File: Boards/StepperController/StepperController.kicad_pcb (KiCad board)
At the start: 2 copper layers, 164 parts, among them IC1 ATMEGA645A-A, J1 I2C, J2 SPI_Extern, J3 ISP, J4 Reference, J5 Display, J7 Spindle, P1 Power, P10 CONN_Z, P2 Cover, P3 USB_B, P4 Relay2, P5 Relay1, P6 Emer_Off, P8 CONN_X, P9 CONN_Y, Q1 BC817-40, Q2 BC817-40, Q3 BC817-40, Q4 BC817-40, Q5 BC817-40, SW2 SW_1, SW3 SW_2, U1 LM2595S-5, U2 74LS11, U3 FT232RL, U5 TMC2660, U6 TMC2660, U7 TMC2660, U8 74HC00, X1 16MHz, Y1 20MHz

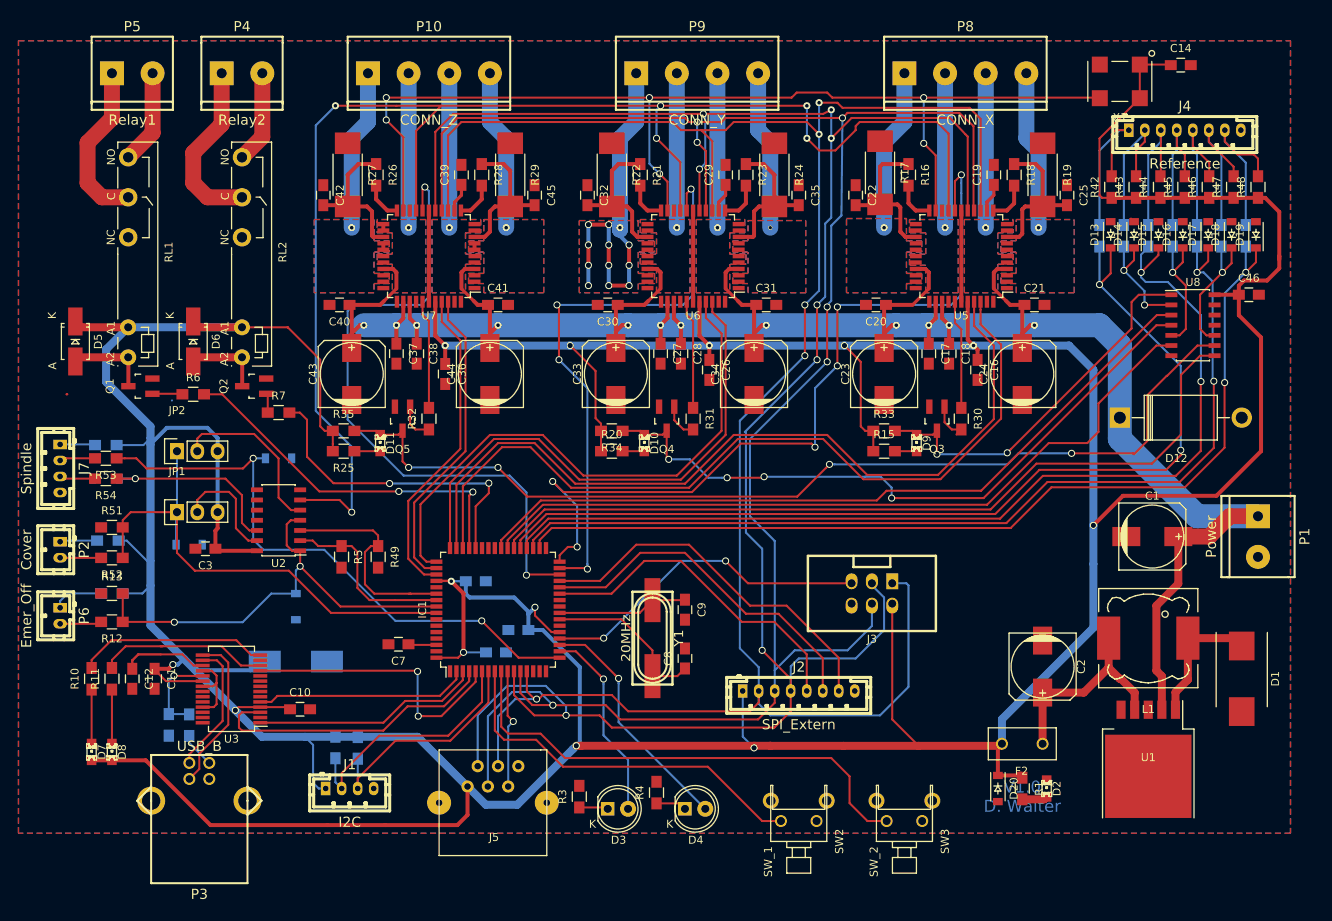
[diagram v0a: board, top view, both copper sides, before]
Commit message: Layouting...
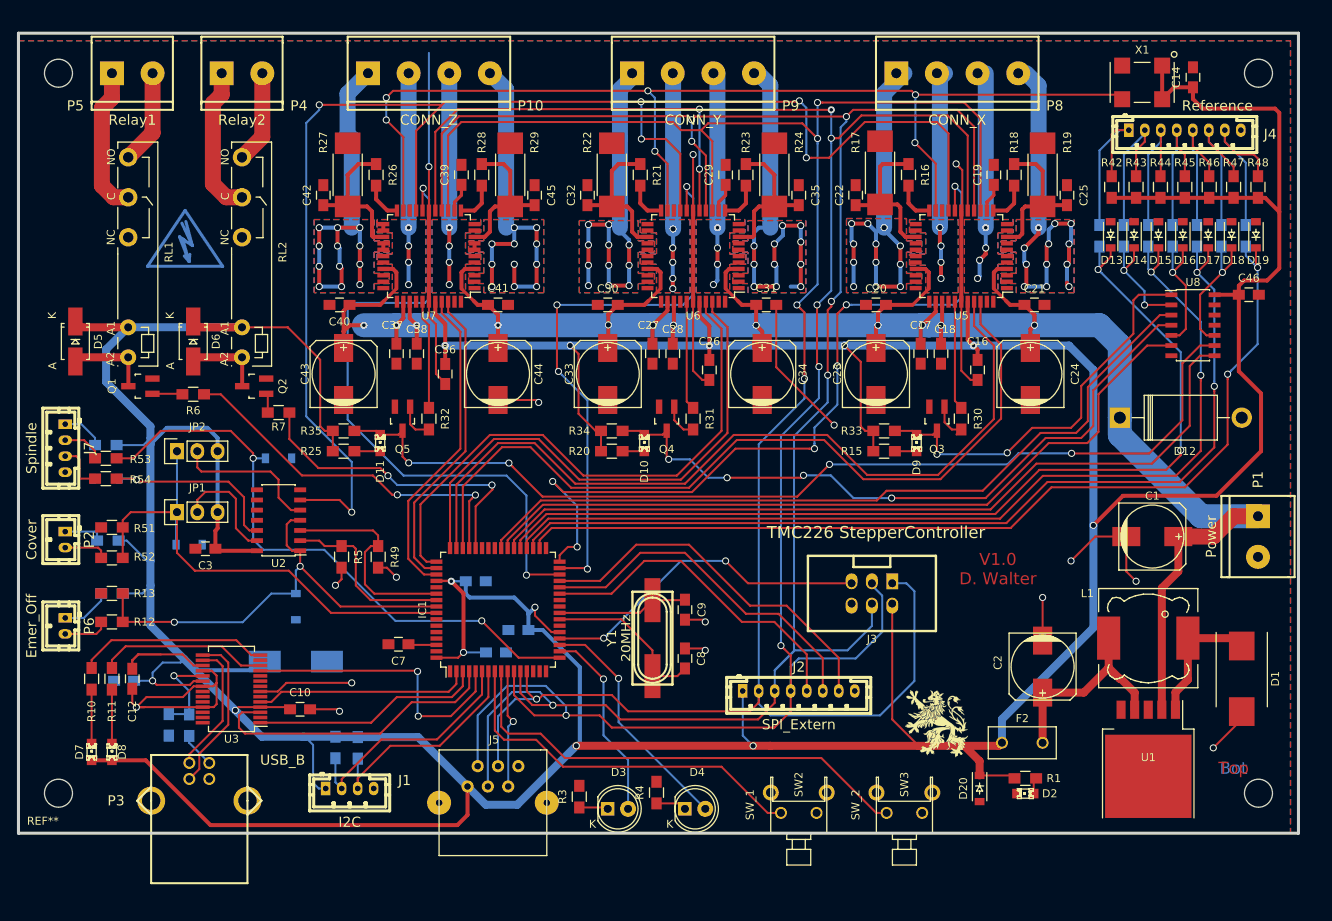
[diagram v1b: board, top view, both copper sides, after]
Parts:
- added G***: LOGO, Loewe:Loewe_Klein, F.Cu at (178.8, 139.2)
- added REF**: EuroBoard160mmX100mm_holes, Euro:EuroBoard160mmX100mm_holes, F.Cu at (64.0, 152.9)
- added REF**: Symbol_HighVoltage_Type2_CopperTop_VerySmall, Symbols:Symbol_HighVoltage_Type2_CopperTop_VerySmall, B.Cu at (84.8, 79.2)
- C11: moved to B.Cu
- moved C11 3.82 mm to (77.2, 133.9), turned to 180 degrees
- moved X1 2.80 mm to (204.5, 59.1)
- moved D2 2.74 mm to (189.9, 148.0), turned to 0 degrees
- moved J7 2.62 mm to (69.8, 104.8)
- moved D20 2.29 mm to (184.2, 147.3)
- moved C14 2.16 mm to (210.8, 58.4), turned to 90 degrees
- moved P2 1.42 mm to (69.8, 116.2)
- moved P6 1.42 mm to (69.8, 127.0)
- moved R1 1.33 mm to (189.9, 146.1), turned to 0 degrees
- moved C17 1.02 mm to (176.8, 93.0)
- moved C28 1.02 mm to (145.8, 93.0)
- moved C34 1.02 mm to (157.0, 95.5)
- moved P8 1.02 mm to (181.4, 57.9)
- moved C43 1.02 mm to (104.6, 95.5)
- moved C18 1.02 mm to (179.3, 93.0)
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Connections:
- net /Driver/Driver_Y/BRN_Y renamed /Driver/Driver_Y/BRB_Y
- R28 pad 2: /Driver/Driver_Z/BRB_Z -> /Driver/Driver_Z/SRA_Z
- U7 pad 12: /Driver/Driver_Z/BRB_Z -> /Driver/Driver_Z/SRA_Z
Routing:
- net GND: track 43.6 -> 207.2 mm, vias 0 -> 16
- net /Driver/Driver_Z/OB1_Z: track 20.9 -> 53.1 mm, vias 1 -> 12
- net /Driver/Driver_Y/OA1_Y: track 19.9 -> 51.1 mm, vias 1 -> 11
- net /Driver/Driver_X/OA1_X: track 19.9 -> 50.2 mm, vias 1 -> 12
- net /Driver/Driver_X/OB1_X: track 20.4 -> 49.9 mm, vias 1 -> 12
- net /Driver/Driver_Z/OA1_Z: track 20.9 -> 47.9 mm, vias 1 -> 11
- net /Driver/Sup_36V: track 309.7 -> 295.4 mm
- net +5V: track 734.7 -> 748.2 mm
- net /Driver/Driver_Y/OB2_Y: track 19.3 -> 27.0 mm, vias 1 -> 5
- net /Driver/Driver_X/TMC_Enable: track 183.0 -> 190.4 mm
- net /Driver/Driver_Y/OA2_Y: track 19.3 -> 26.6 mm, vias 1 -> 4
- net /Driver/Driver_Z/OB2_Z: track 20.1 -> 27.2 mm, vias 1 -> 4
- net /Driver/Driver_Z/OA2_Z: track 19.3 -> 26.4 mm, vias 1 -> 4
- net /Driver/Driver_X/OA2_X: track 19.3 -> 26.1 mm, vias 1 -> 4
- net /Driver/Driver_X/OB2_X: track 19.3 -> 26.0 mm, vias 1 -> 4
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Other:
- board outline added: 160 x 100 mm
- board text added: "Bot"
- board text added: "TMC226 StepperController"
- board text added: "Top"
